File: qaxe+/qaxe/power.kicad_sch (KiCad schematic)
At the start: 74 parts, among them Q3 CSD16415Q5T, Q4 CSD16415Q5T, Q7 CSD16415Q5T, Q8 CSD16415Q5T, U17 LTC3856, U2 +0V8, U3 AP3211, U36 1117-3.3, U4 MCP1824T-0802E, U5 +0V8, U7 MCP1824T-1802E

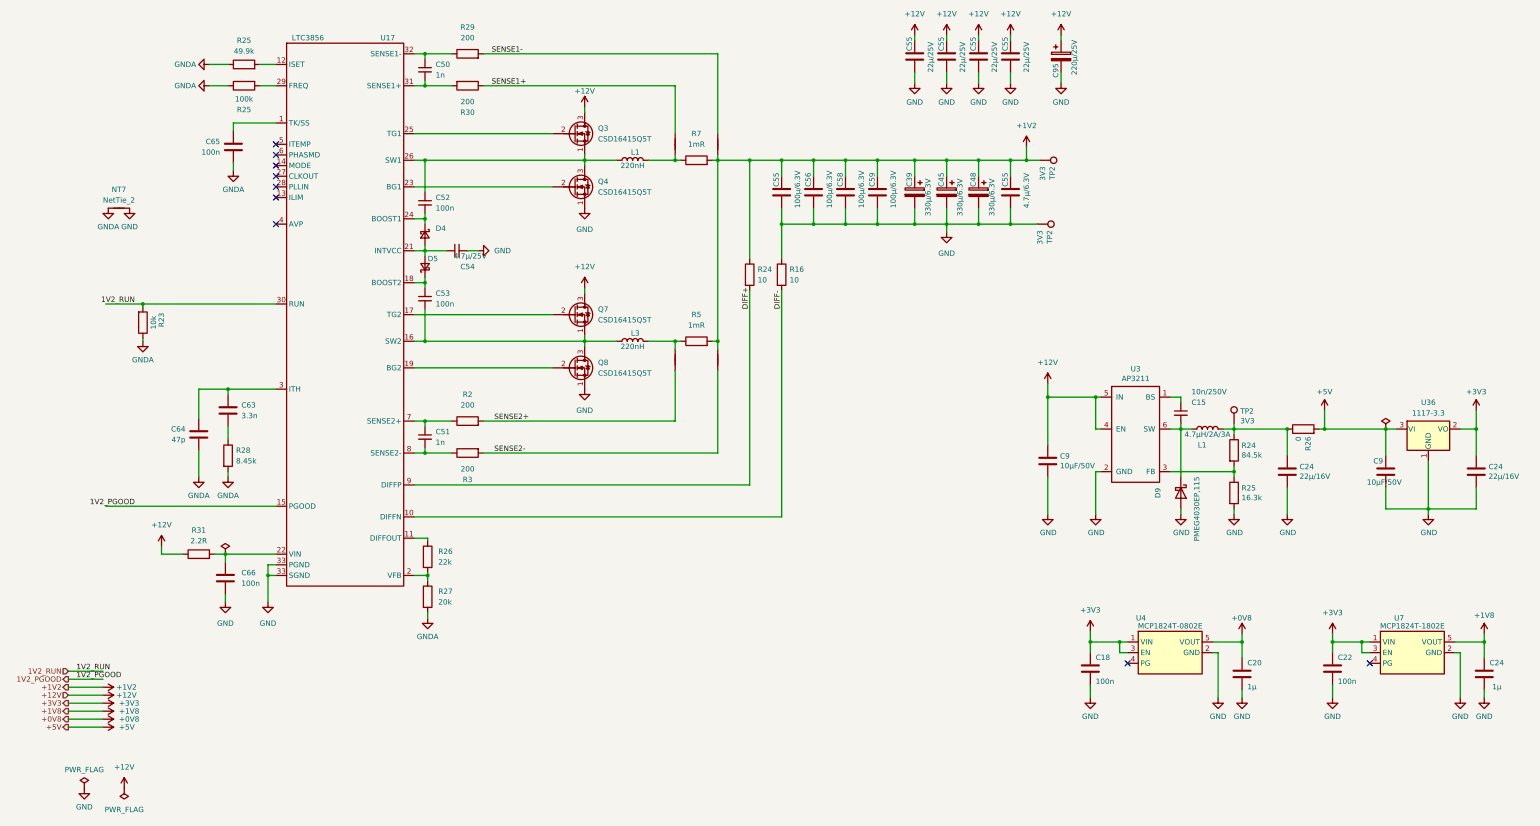
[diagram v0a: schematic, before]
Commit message: qaxe+
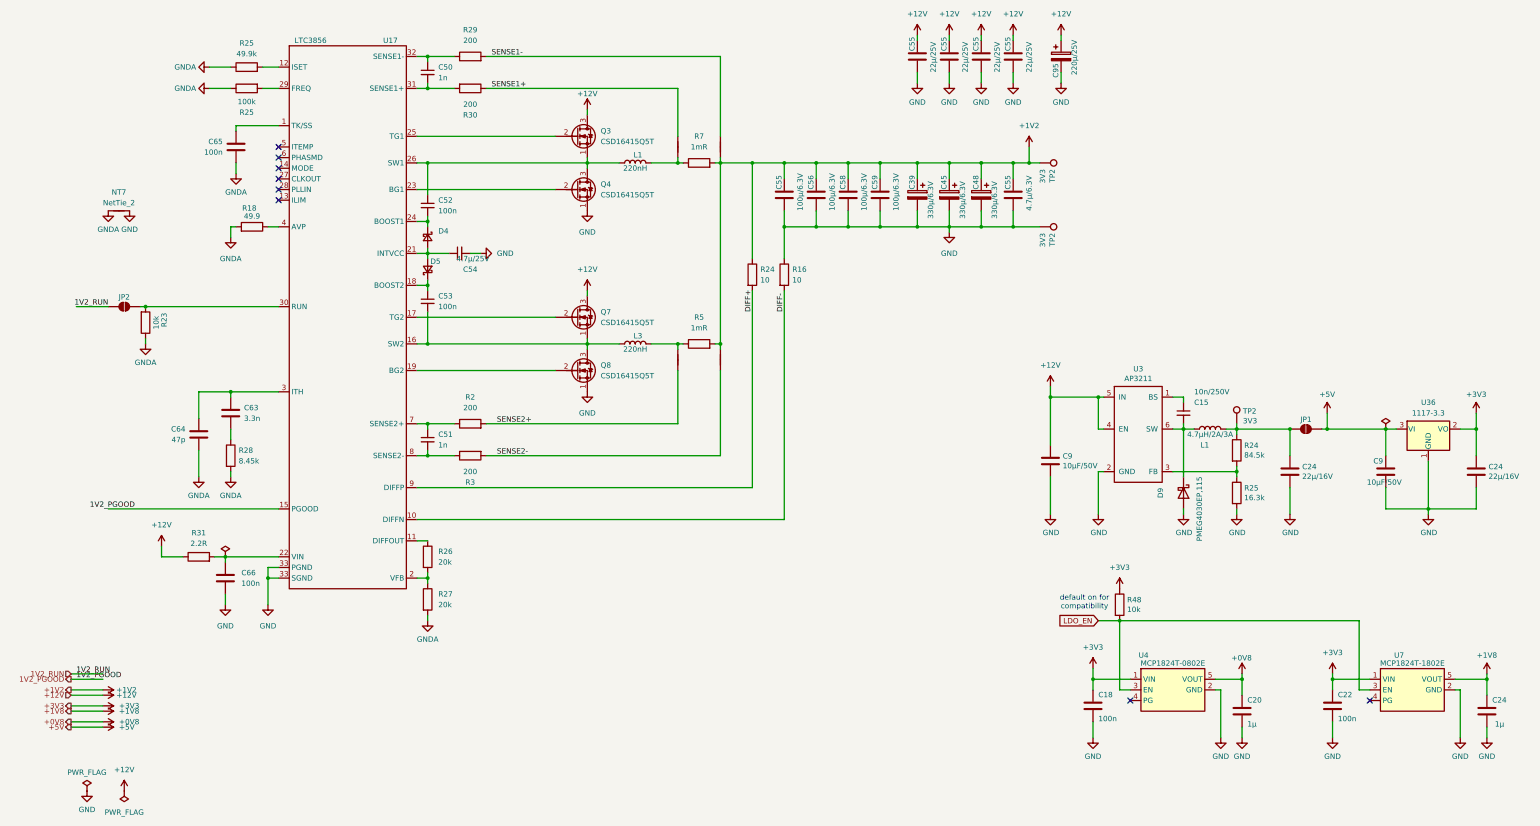
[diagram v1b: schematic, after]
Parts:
- removed R26: 0, Resistor_SMD:R_1210_3225Metric, symbol Device:R
- added JP1, JP2: SolderJumper_2_Open, Jumper:SolderJumper-2_P1.3mm_Open_RoundedPad1.0x1.5mm, symbol Jumper:SolderJumper_2_Open
- added R18: 49.9, Resistor_SMD:R_0805_2012Metric, symbol Device:R
- added R48: 10k, Resistor_SMD:R_0805_2012Metric, symbol Device:R
- R26: value 22k -> 20k
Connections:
- net +3V3: now also R48.1; no longer U4.3 (EN), U7.3 (EN)
- net +5V: now also JP1.2 (B)
- net 1V2_RUN: now also JP2.1 (A); no longer R23.2, U17.30 (RUN)
- net GNDA: now also R18.2
- net at C24.1, L1.2, R24.1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: now also JP1.1 (A)
- net at U17.4 (AVP): now also R18.1
- new net: JP2.2 (B), R23.2, U17.30 (RUN)
- new net LDO_EN: R48.2, U4.3 (EN), U7.3 (EN)
- no-connect marks 9 -> 8
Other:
- note added: "default on for compatibility"
- moved on the sheet: C15, C18, C20, C22, C24, C39, C45, C48, C50, C51, C52, C53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

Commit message: some bom fixes
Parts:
- TP2: now left out of the parts list
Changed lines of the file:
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@@
 		(unit 1)
 		(exclude_from_sim no)
-		(in_bom yes)
+		(in_bom no)
 		(on_board yes)
 		(dnp no)
